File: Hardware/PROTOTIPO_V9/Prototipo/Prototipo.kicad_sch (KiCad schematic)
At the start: 1 part, among them U3 YAAJ_BlackPill_Part_Like_SWD_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

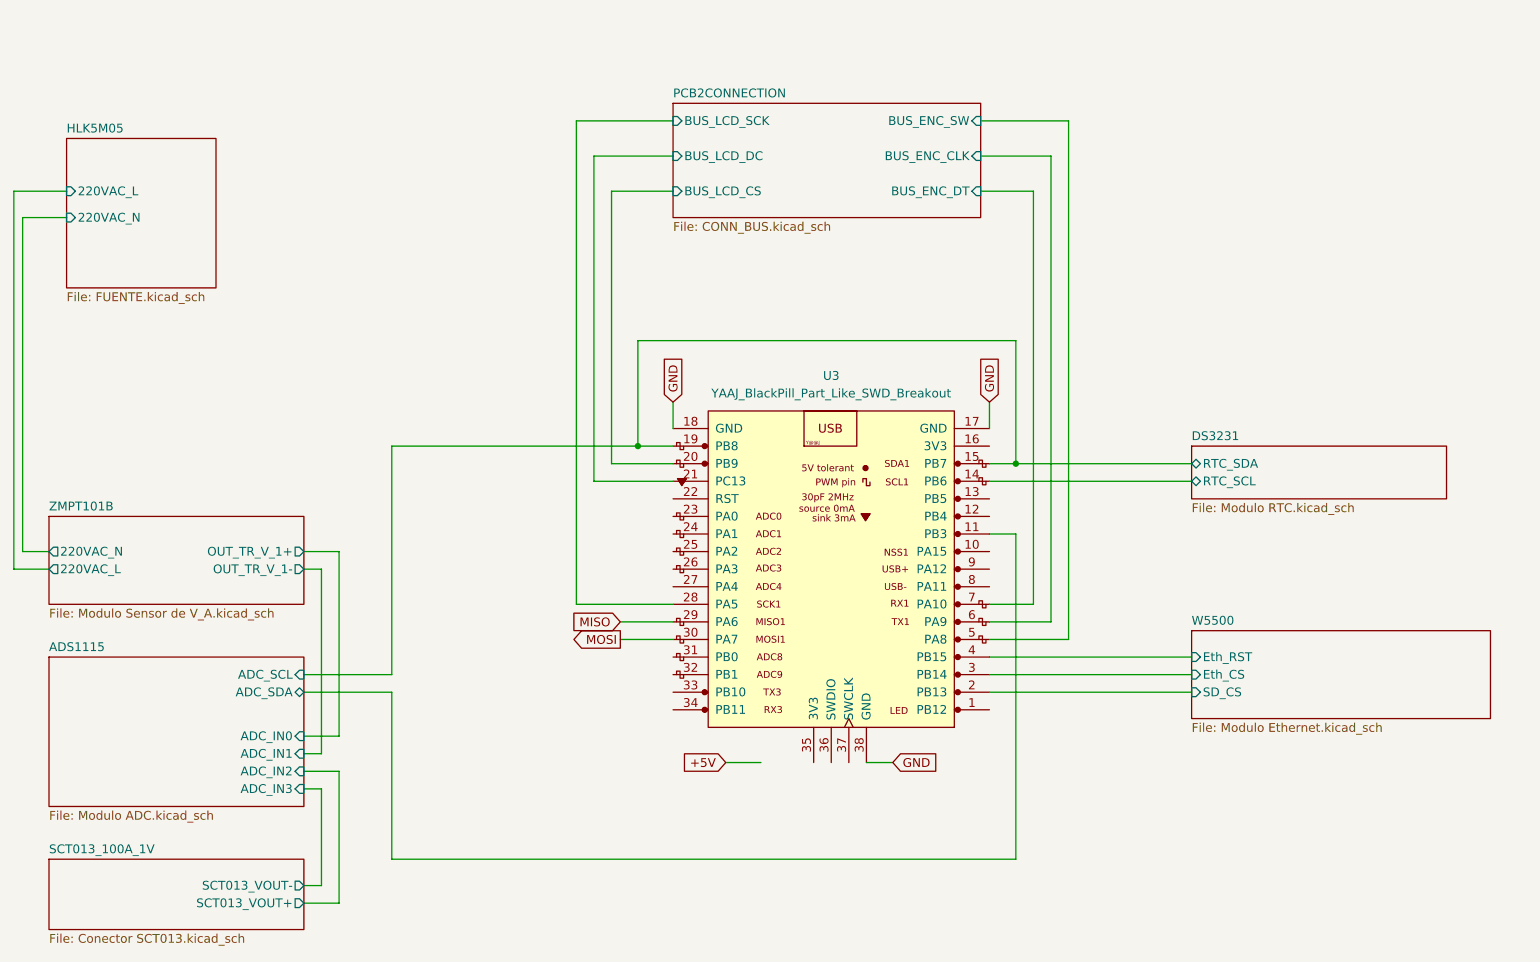
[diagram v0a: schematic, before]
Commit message: Shc final y ruteo de PCB
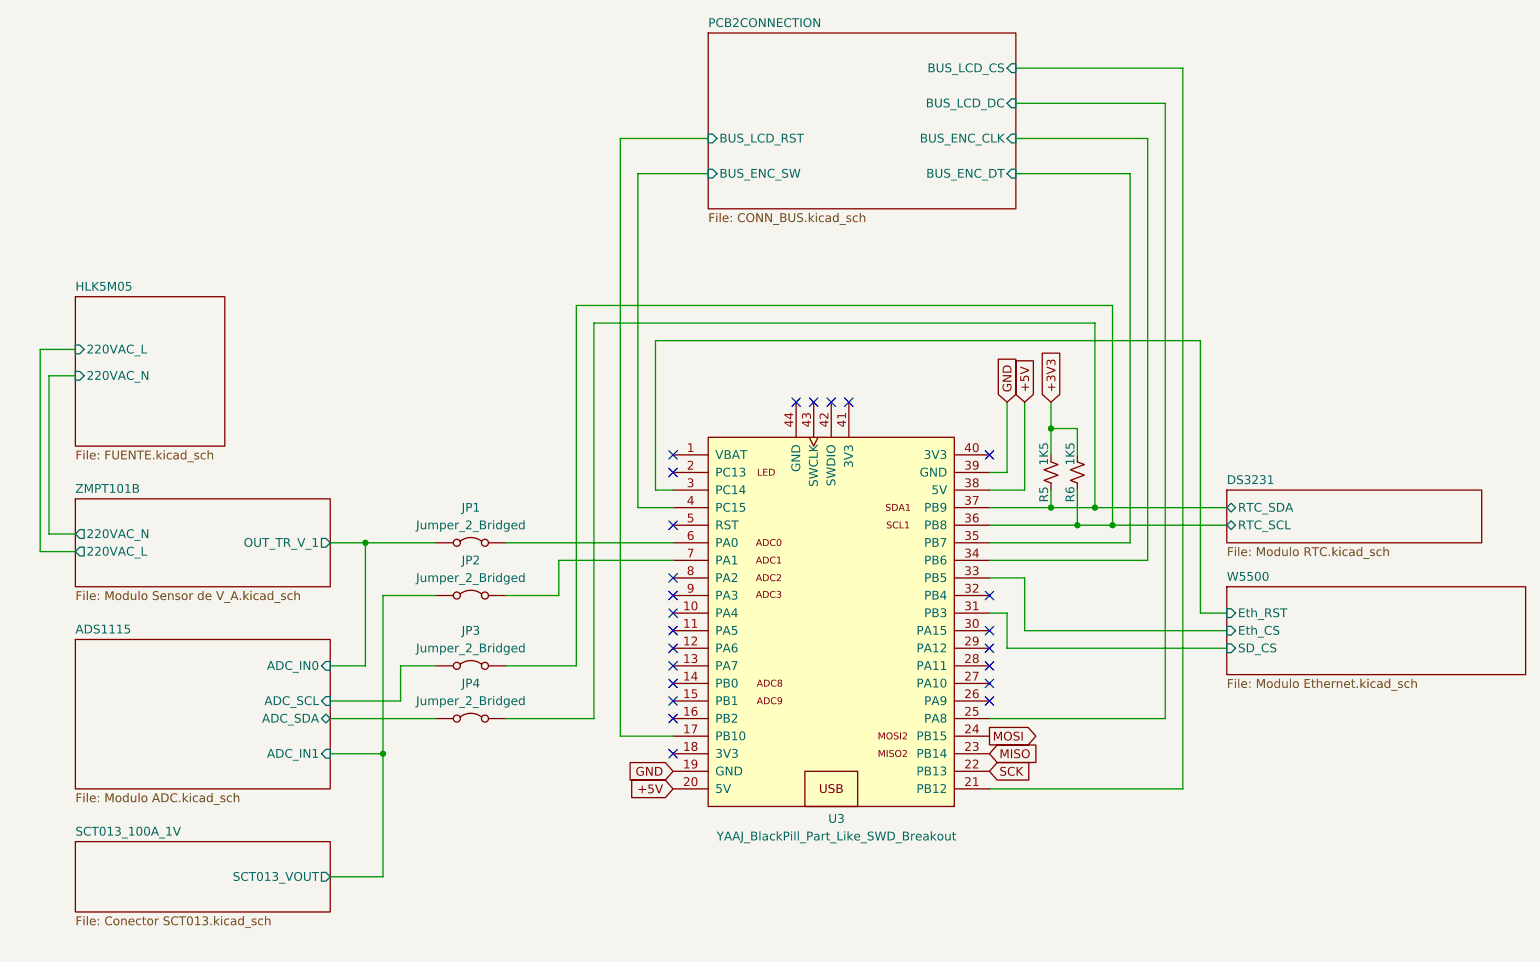
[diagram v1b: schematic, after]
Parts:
- added JP1, JP2, JP3, JP4: Jumper_2_Bridged, Connector_PinHeader_2.54mm:PinHeader_1x02_P2.54mm_Vertical, symbol Jumper:Jumper_2_Bridged
- added R5, R6: 1K5, Resistor_THT:R_Axial_DIN0207_L6.3mm_D2.5mm_P10.16mm_Horizontal, symbol Device:R_Small_US
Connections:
- net +5V: now also U3.20 (5V), U3.38 (5V)
- net ADS1115/ADC_IN0: now also JP1.1 (A)
- net ADS1115/ADC_IN1: now also JP2.1 (A)
- net ADS1115/ADC_SCL: now also JP3.1 (A); no longer U3.15 (PB7), U3.19 (PB8)
- net ADS1115/ADC_SDA: now also JP4.1 (A); no longer U3.11 (PB3)
- net DS3231/RTC_SCL: now also U3.36 (PB8), JP3.2 (B), R6.2; no longer U3.14 (PB6)
- net GND: now also U3.19 (GND), U3.39 (GND); no longer U3.17 (GND), U3.18 (GND), U3.38 (GND)
- net MISO: now also U3.23 (PB14); no longer U3.29 (PA6)
- net MOSI: now also U3.24 (PB15); no longer U3.30 (PA7)
- net PCB2CONNECTION/BUS_ENC_CLK: now also U3.34 (PB6); no longer U3.6 (PA9)
- net PCB2CONNECTION/BUS_ENC_DT: now also U3.35 (PB7); no longer U3.7 (PA10)
- net PCB2CONNECTION/BUS_ENC_SW: now also U3.4 (PC15); no longer U3.5 (PA8)
- net PCB2CONNECTION/BUS_LCD_CS: now also U3.21 (PB12); no longer U3.20 (PB9)
- net PCB2CONNECTION/BUS_LCD_DC: now also U3.25 (PA8); no longer U3.21 (PC13)
- net W5500/Eth_CS: now also U3.33 (PB5); no longer U3.3 (PB14)
- net W5500/Eth_RST: now also U3.3 (PC14); no longer U3.4 (PB15)
- net W5500/SD_CS: now also U3.31 (PB3); no longer U3.2 (PB13)
- net SCK: now reaches U3.22 (PB13)
- net DS3231/RTC_SDA: now reaches U3.37 (PB9)
- net DS3231/RTC_SDA: now also JP4.2 (B), R5.2
- net PCB2CONNECTION/BUS_LCD_SCK: no longer names the net of U3.28 (PA11)
- new net: JP1.2 (B), U3.6 (PA0)
- new net: JP2.2 (B), U3.7 (PA1)
- new net +3V3: R5.1, R6.1
- new net PCB2CONNECTION/BUS_LCD_RST: U3.17 (PB10)
- no-connect marks 0 -> 24
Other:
- sheet ADS1115 ports: added none; removed ADC_IN2, ADC_IN3
- sheet PCB2CONNECTION ports: added BUS_LCD_RST; removed BUS_LCD_SCK
- sheet SCT013_100A_1V ports: added SCT013_VOUT; removed SCT013_VOUT+, SCT013_VOUT-
- sheet ZMPT101B ports: added OUT_TR_V_1; removed OUT_TR_V_1+, OUT_TR_V_1-
